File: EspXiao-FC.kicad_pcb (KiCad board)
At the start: 2 copper layers, 33 x 33 mm, 11 parts, among them J1 Conn_01x08_Pin, J2 Conn_01x02_Pin, J3 Conn_01x02_Pin, J4 Conn_01x02_Pin, J5 Conn_01x02_Pin, J6 Conn_01x02_Pin, Q1 IRFZ44N, Q2 IRFZ44N, Q3 IRFZ44N, Q4 IRFZ44N, U1 MOUDLE-SEEEDUINO-XIAO-ESP32S3

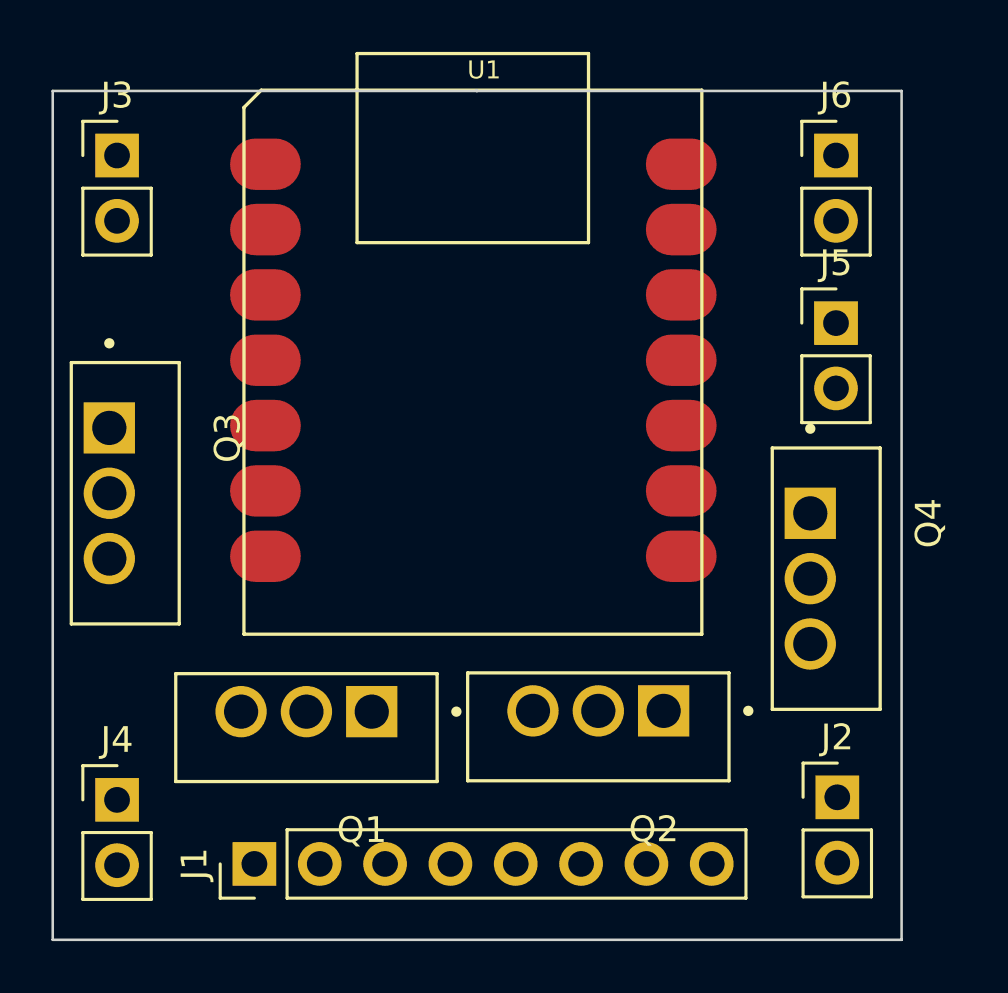
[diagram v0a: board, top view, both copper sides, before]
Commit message: Complete
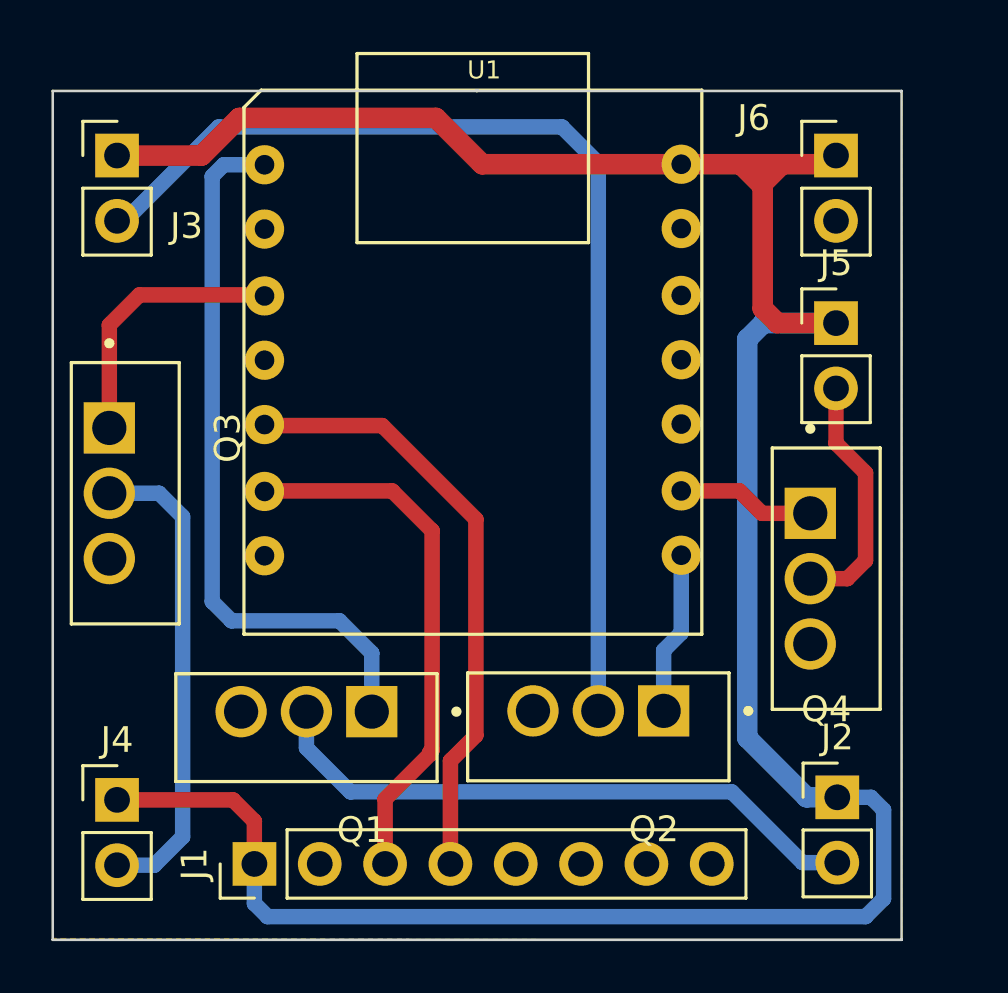
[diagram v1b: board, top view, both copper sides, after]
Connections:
- J1 pad 1: MotorA -> VCC
- J2 pad 1: MotorA -> VCC
- J2 pad 2: GNDREF -> MotorA
- J3 pad 1: MotorA -> VCC
- J3 pad 2: GNDREF -> MotorB
- J4 pad 1: MotorA -> VCC
- J4 pad 2: GNDREF -> MotorC
- J5 pad 1: MotorA -> VCC
- J5 pad 2: GNDREF -> MotorD
- J6 pad 1: MotorA -> VCC
- Q2 pad 2: MotorA -> MotorB
- Q3 pad 2: MotorA -> MotorC
- Q4 pad 2: MotorA -> MotorD
- U1 pad 14: MotorA -> VCC
- U1 pad 2: MOTOR_B_PWM -> unconnected-(U1-PA4_A1_D1-Pad2)
- U1 pad 4: MOTOR_D_PWM -> unconnected-(U1-PA11_A3_D3-Pad4)
- U1 pad 8: unconnected-(U1-PB09_D7_RX-Pad8) -> MOTOR_B_PWM
- U1 pad 9: unconnected-(U1-PA7_A8_D8_SCK-Pad9) -> MOTOR_D_PWM
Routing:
- net VCC: track 0.00 -> 103.5 mm
- net MotorB: track 0.00 -> 42.1 mm
- net MOTOR_A_PWM: track 0.00 -> 28.1 mm
- net MotorA: track 0.00 -> 23.9 mm
- net SDA: track 0.00 -> 23.5 mm
- net SCL: track 0.00 -> 20.8 mm
- net MotorC: track 0.00 -> 18.7 mm
- net MOTOR_C_PWM: track 0.00 -> 10.6 mm
- net MotorD: track 0.00 -> 9.61 mm
- net MOTOR_B_PWM: track 0.00 -> 6.33 mm
- net MOTOR_D_PWM: track 0.00 -> 5.38 mm
- added copper zone on F.Cu, net GNDREF
